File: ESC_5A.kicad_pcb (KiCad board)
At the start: 2 copper layers, 39 parts, among them IC1 EEPROM, IC2 3.3V Reg, IC3 5V_Reg, IC4 ATSAMD21E17D-AUT, J1 USBc, J2 5V_PWR, J3 M1, J4 M2, J5 PWR_IN, U1 TB67H420FTG_EL

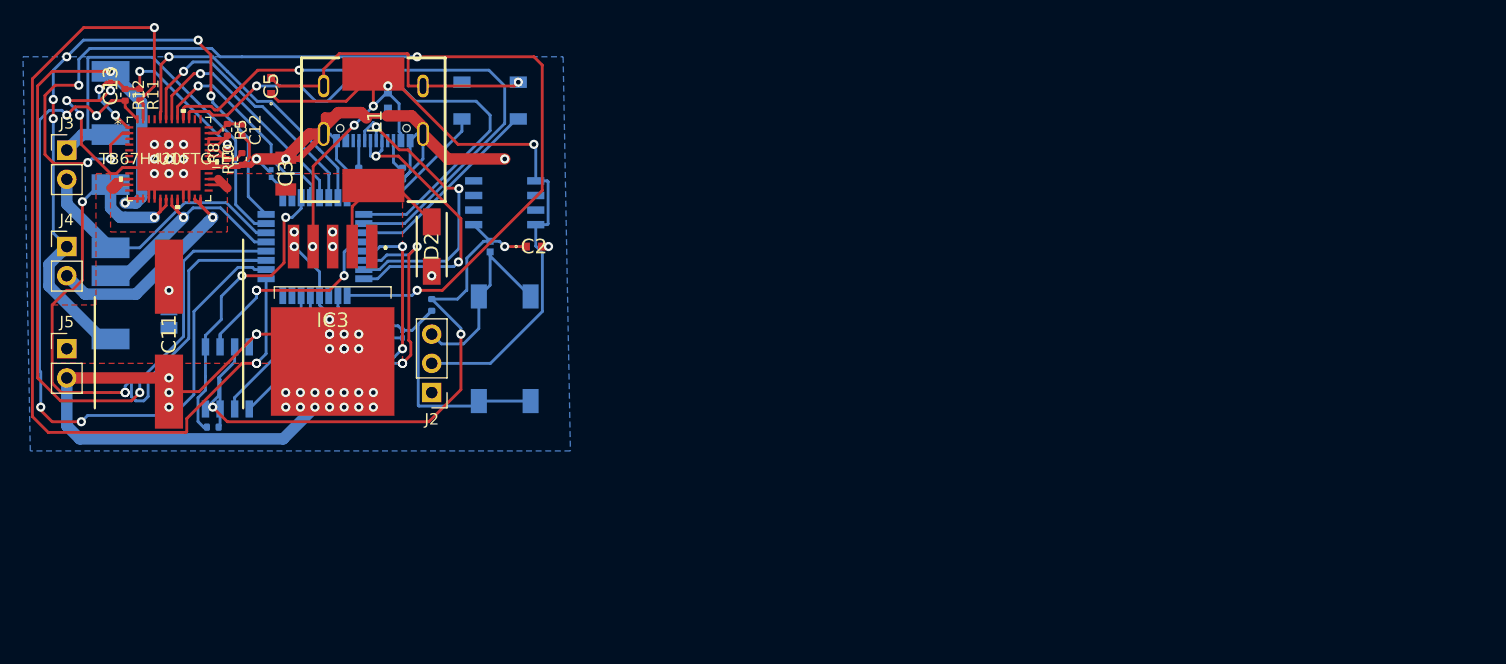
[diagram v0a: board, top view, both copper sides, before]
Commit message: feather profile
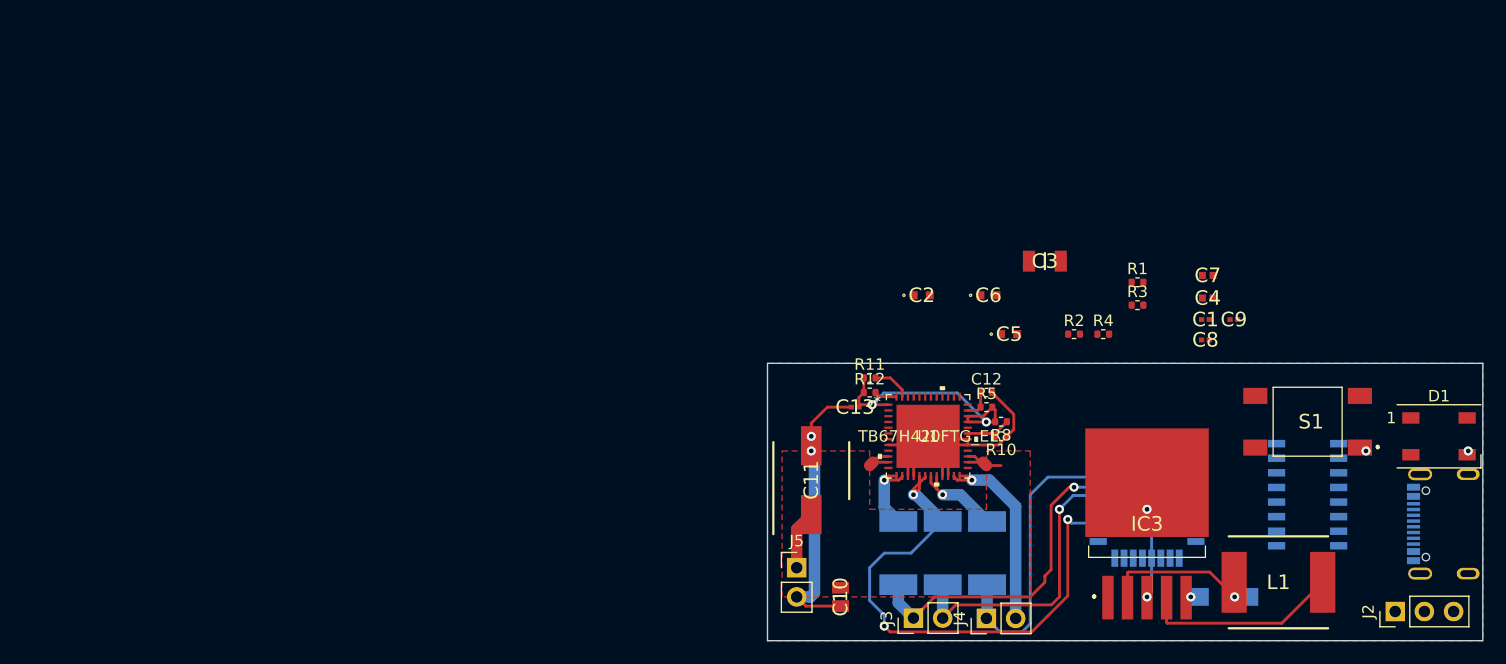
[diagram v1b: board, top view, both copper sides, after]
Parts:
- C1, C10, C4, C6, C7, C8, C9, D1, R1, R2, R3, R4, S1: moved to F.Cu
- C11: footprint SamacSys_Parts:CAPAE1290X1650N -> SamacSys_Parts:CAPAE660X800N
- D2: moved to B.Cu
- L1: footprint SamacSys_Parts:SRR1260-150M -> SamacSys_Parts:INDM8680X300N
- moved J1 102.6 mm to (278.1, 59.7), turned to 270 degrees
- moved IC1 94.3 mm to (264.2, 54.6), turned to 0 degrees
- moved L1 88.0 mm to (261.6, 64.8), turned to 0 degrees
- moved D1 87.6 mm to (275.6, 52.1)
- moved J4 86.3 mm to (236.2, 67.9), turned to 90 degrees
- moved J2 86.0 mm to (271.8, 67.3), turned to 90 degrees
- moved C9 84.7 mm to (257.7, 41.9), turned to 0 degrees
- moved J3 84.2 mm to (229.9, 67.9), turned to 90 degrees
- moved R6 79.2 mm to (236.3, 62.2)
- moved R7 78.9 mm to (228.6, 62.2)
- moved C8 78.8 mm to (255.3, 43.7), turned to 0 degrees
- moved R9 78.1 mm to (232.4, 62.2)
- moved R4 77.9 mm to (246.4, 43.2), turned to 0 degrees
- moved C7 77.8 mm to (255.5, 38.1), turned to 0 degrees
- moved IC4 75.9 mm to (250.2, 58.4)
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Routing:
- net GND: track 225.4 -> 70.8 mm, vias 50 -> 7
- net HBMODE: track 93.8 -> 0.00 mm, vias 5 -> 0
- net LO1: track 81.4 -> 3.35 mm, vias 3 -> 0
- net ADC_VREFA: track 79.0 -> 7.06 mm, vias 3 -> 1
- net LO2: track 66.8 -> 1.97 mm, vias 4 -> 0
- net +5V: track 81.4 -> 17.2 mm, vias 5 -> 0
- net +3V3: track 58.6 -> 0.00 mm, vias 3 -> 0
- net PWMB: track 52.6 -> 0.00 mm, vias 1 -> 0
- net PWMA: track 46.1 -> 0.00 mm, vias 1 -> 0
- net ADC_2: track 58.5 -> 25.3 mm, vias 5 -> 0
- net MOSI_EEPROM: track 31.0 -> 0.00 mm, vias 3 -> 0
- net SCK_EEPROM: track 29.8 -> 0.00 mm, vias 2 -> 0
- net NRST: track 29.4 -> 0.00 mm
- net D-: track 27.6 -> 0.00 mm, vias 2 -> 0
- net INB2: track 27.6 -> 0.00 mm, vias 1 -> 0
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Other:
- board outline added: 62.2 x 24.1 mm
